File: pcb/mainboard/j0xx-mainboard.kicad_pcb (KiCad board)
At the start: 2 copper layers, 67.5 x 63.2 mm, 33 parts, among them J1 USB_C_Receptacle, J2 Conn_01x08, J3 Conn_01x06, J4 Conn_01x05, J5 Conn_01x09, J6 Conn_01x11, Q1 BSS138, SW1 reset, U1 ATmega32U4-AU, Y1 Resonator

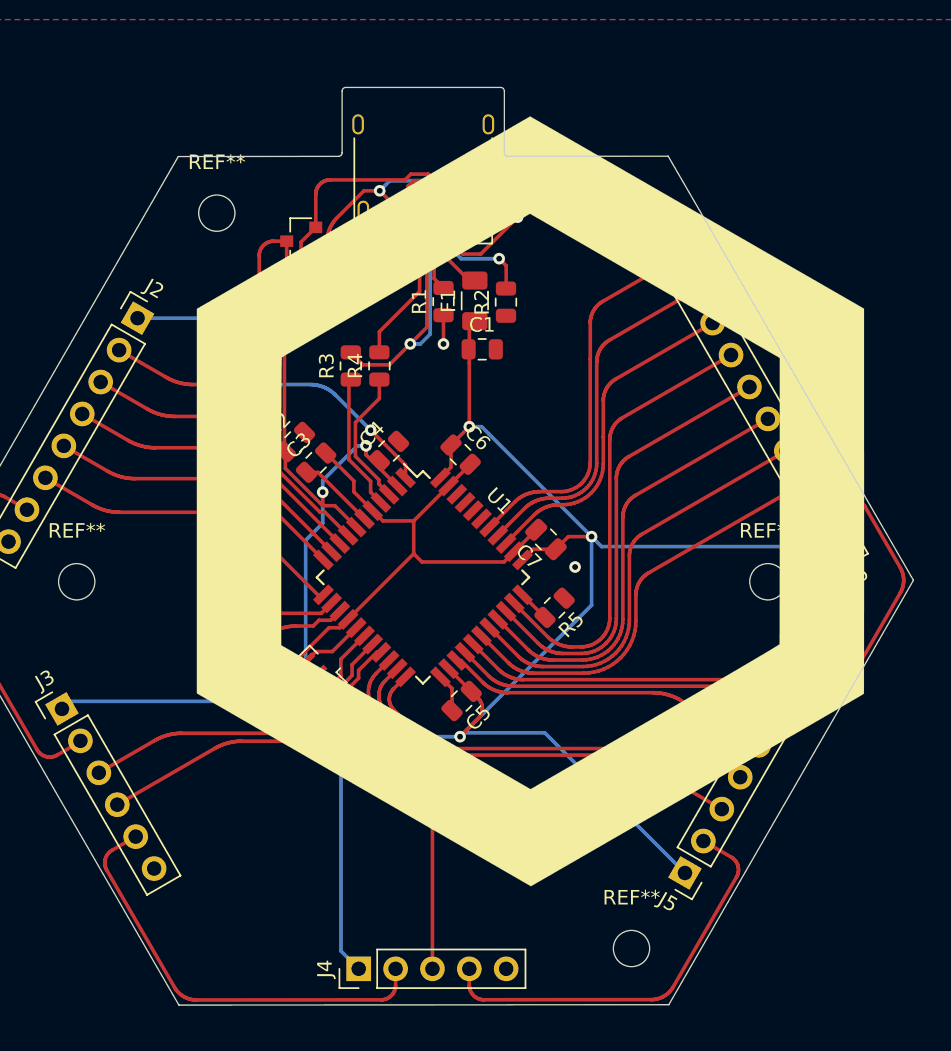
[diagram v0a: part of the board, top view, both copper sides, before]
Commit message: First full iteration of physical design
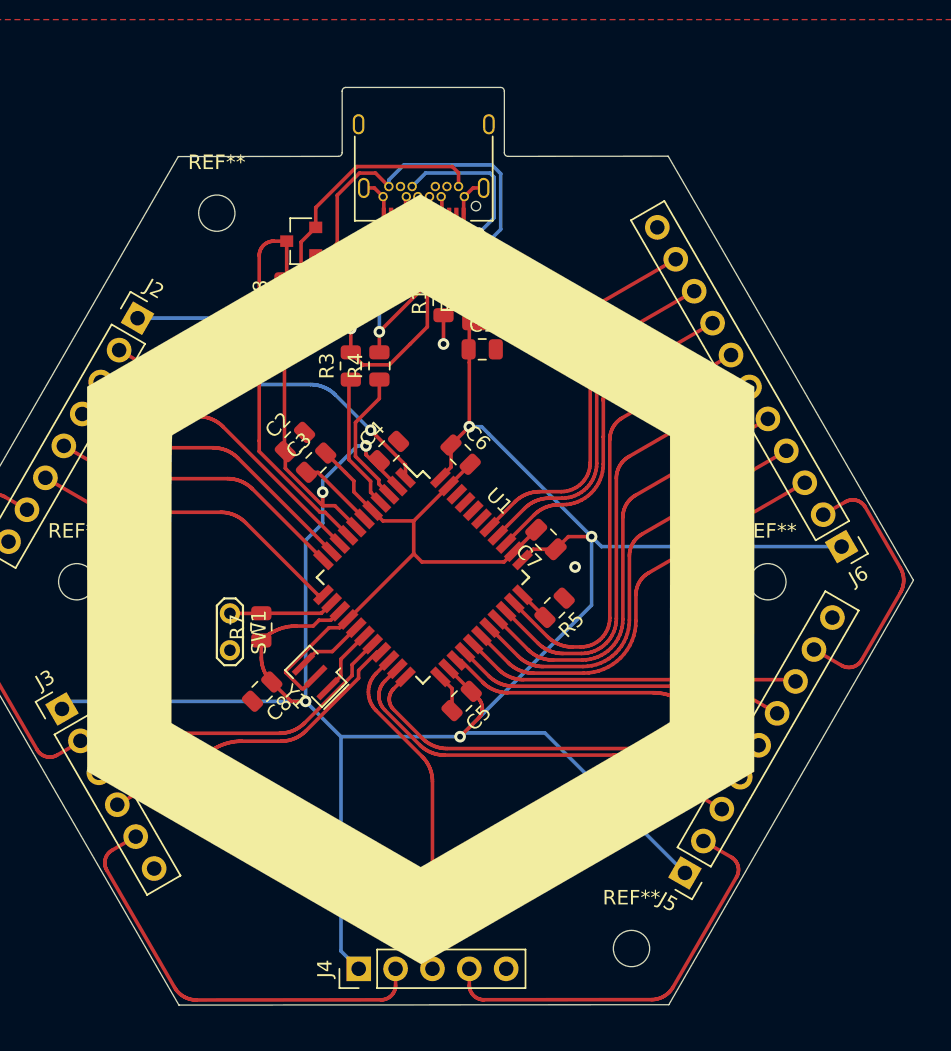
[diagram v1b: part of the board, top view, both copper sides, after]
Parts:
- J1: footprint Connector_USB:USB_C_Receptacle_Amphenol_12401610E4-2A -> USB_C:USB_C_LCSC_C456013
- Y1: footprint Crystal:Resonator_SMD_muRata_CSTxExxV-3Pin_3.0x1.1mm -> Crystal:Resonator_SMD_Murata_CSTxExxV-3Pin_3.0x1.1mm
- moved G*** 9.28 mm to (204.2, 98.1)
- moved G*** 9.26 mm to (204.2, 98.1)
- moved J1 4.58 mm to (207.8, 72.5)
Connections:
- J1 pad A10: Net-(J1-PadA10) -> unconnected-(J1-PadA10)
- J1 pad A3: Net-(J1-PadA3) -> unconnected-(J1-PadA3)
- J1 pad A8: Net-(J1-PadA8) -> unconnected-(J1-PadA8)
- J1 pad B10: Net-(J1-PadB10) -> unconnected-(J1-PadB10)
- J1 pad B3: Net-(J1-PadB3) -> unconnected-(J1-PadB3)
- J1 pad B8: Net-(J1-PadB8) -> unconnected-(J1-PadB8)
- U1 pad 39: Net-(U1-Pad39) -> unconnected-(U1-Pad39)
- U1 pad 40: Net-(U1-Pad40) -> unconnected-(U1-Pad40)
- U1 pad 41: Net-(U1-Pad41) -> unconnected-(U1-Pad41)
- U1 pad 42: Net-(U1-Pad42) -> unconnected-(U1-Pad42)
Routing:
- net D-: track 11.2 -> 22.1 mm, vias 0 -> 1
- net GND: track 55.7 -> 51.7 mm
- net D+: track 24.8 -> 28.7 mm, vias 2 -> 1
- net Net-(F1-Pad2): track 13.5 -> 17.4 mm, vias 0 -> 2
- net Net-(J1-PadB5): track 13.3 -> 15.2 mm, vias 2 -> 1
- net Net-(J1-PadA5): track 3.68 -> 5.35 mm
- net +3V3: track 27.6 -> 29.1 mm, vias 2 -> 1
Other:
- net class Default removed
